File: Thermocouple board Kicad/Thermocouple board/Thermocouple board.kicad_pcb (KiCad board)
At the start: 2 copper layers, 83 parts, among them J1 Conn_01x06_Pin, J2 Conn_01x02_Pin, Q2 2N3904, Q3 2N3904, U1 LTC2984CLX-PBF

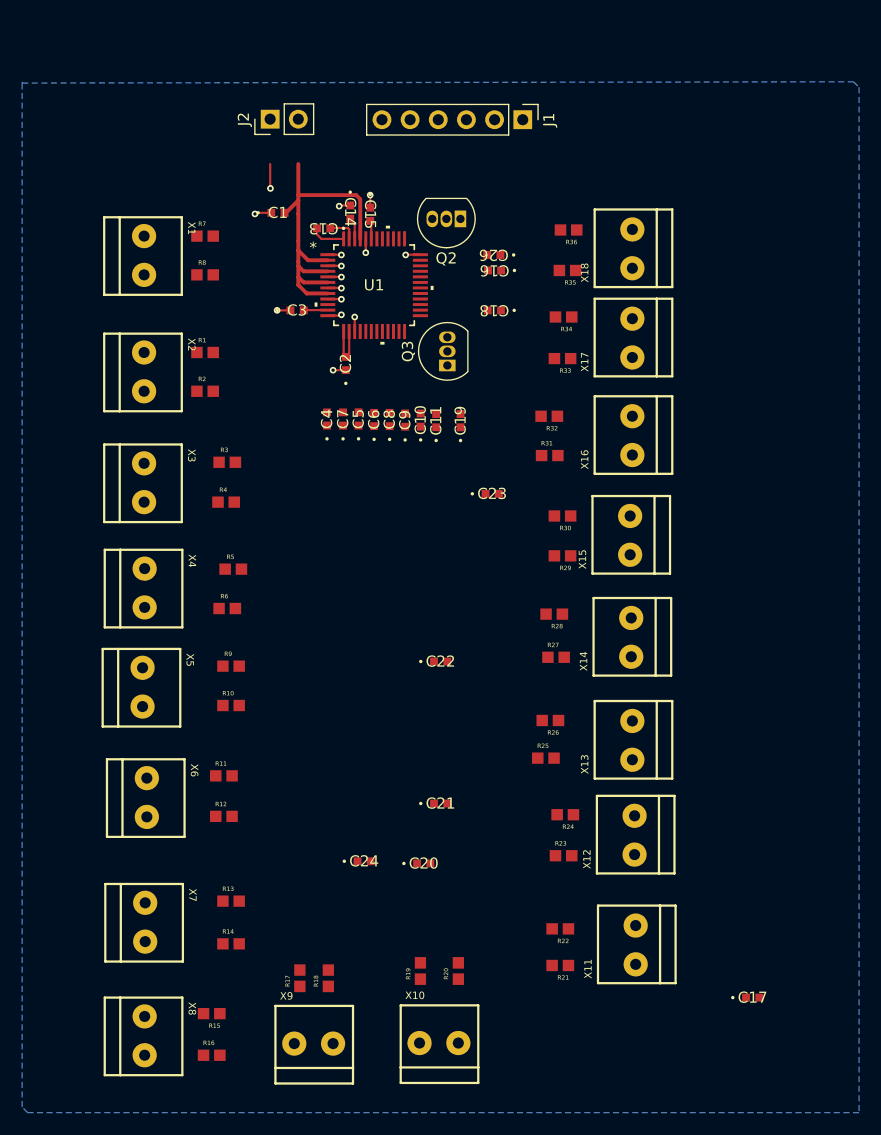
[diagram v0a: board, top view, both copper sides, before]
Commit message: Add files via upload
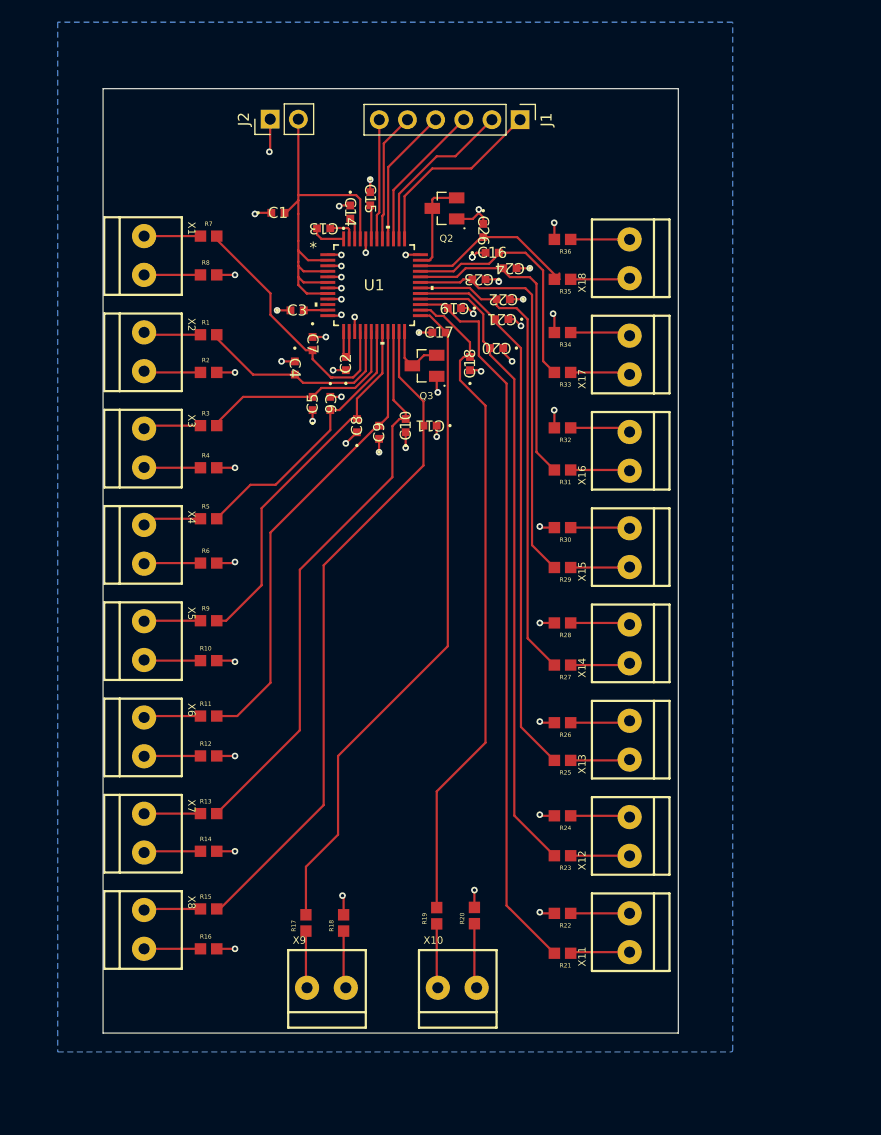
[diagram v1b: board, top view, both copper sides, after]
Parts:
- Q2, Q3: footprint Package_TO_SOT_THT:TO-92_Inline -> BJT:SOT95P240X111-3N
- moved C17 66.3 mm to (123.6, 60.2)
- moved C24 55.1 mm to (130.0, 54.4), turned to 180 degrees
- moved C20 47.0 mm to (128.8, 61.6), turned to 180 degrees
- moved C21 44.0 mm to (129.3, 59.0), turned to 180 degrees
- moved C22 33.2 mm to (129.4, 57.2), turned to 180 degrees
- moved C23 19.4 mm to (127.2, 55.4), turned to 180 degrees
- moved C19 10.2 mm to (125.0, 58.0), turned to 180 degrees
- moved R16 9.60 mm to (102.8, 115.8)
- moved X8 9.60 mm to (97.0, 114.0)
- moved R15 9.45 mm to (102.8, 112.2), turned to 0 degrees
- moved R14 8.59 mm to (102.8, 107.0)
- moved R13 8.16 mm to (102.8, 103.6)
- moved X7 8.04 mm to (97.0, 105.3)
- moved C7 7.34 mm to (112.2, 61.2), turned to -90 degrees
- moved R12 5.62 mm to (102.8, 98.4)
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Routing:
- net /Channel12: track 0.00 -> 65.8 mm
- net /Channel10: track 0.00 -> 60.9 mm
- net /Channel8: track 0.00 -> 60.6 mm
- net /Channel11: track 0.00 -> 60.1 mm
- net /Channel13: track 0.00 -> 57.8 mm
- net GND: track 19.6 -> 74.8 mm, vias 15 -> 53
- net /Channel7: track 0.00 -> 51.3 mm
- net /Channel14: track 0.00 -> 49.7 mm
- net /Channel15: track 0.00 -> 43.4 mm
- net /Channel6: track 0.00 -> 42.1 mm
- net /Channel16: track 0.00 -> 36.3 mm
- net /Channel5: track 0.00 -> 32.9 mm
- net /Channel17: track 0.00 -> 29.0 mm
- net /Channel4: track 0.00 -> 24.7 mm
- net /Channel1: track 0.00 -> 24.1 mm
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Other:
- board outline added: 51.9 x 85.2 mm
